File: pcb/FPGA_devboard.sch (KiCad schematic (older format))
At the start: 4 parts

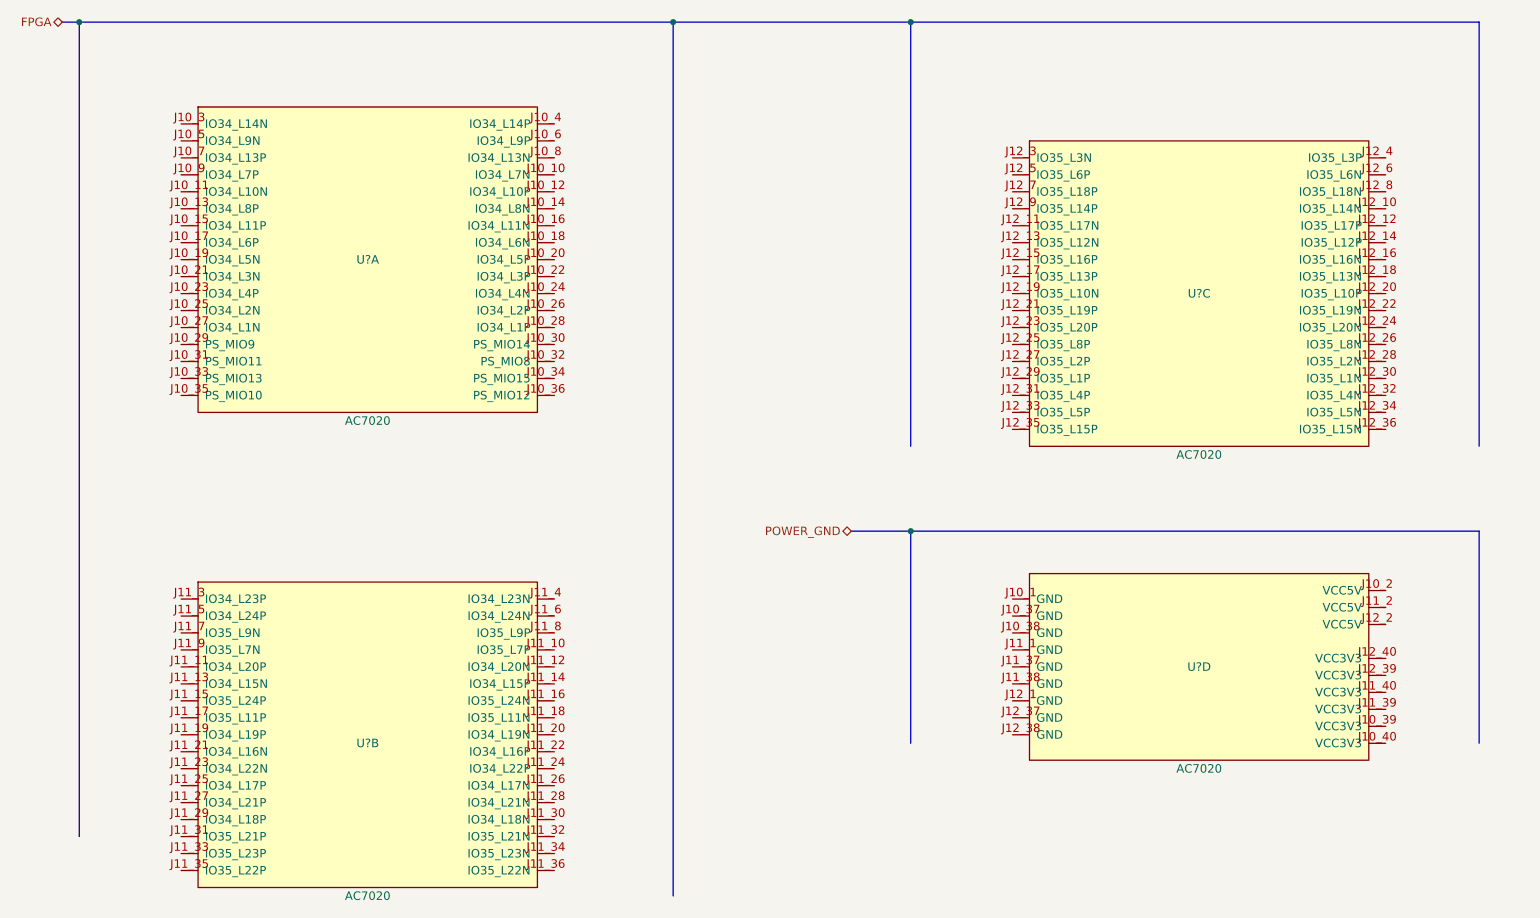
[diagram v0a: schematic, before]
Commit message: Some work done on the whole project
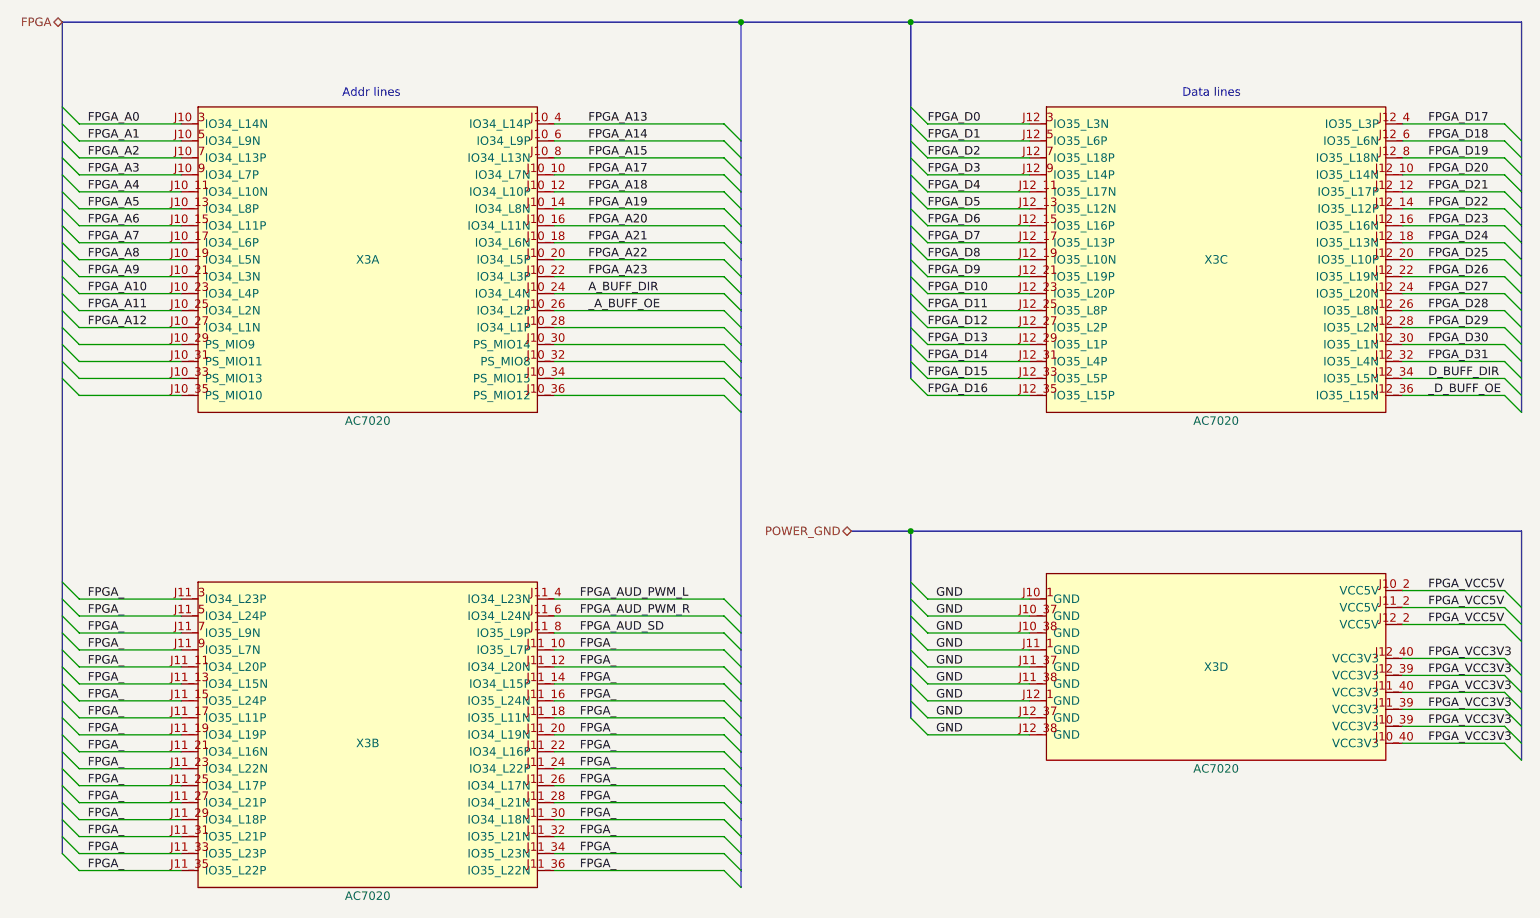
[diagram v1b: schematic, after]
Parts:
- gave numbers to parts that had none: 1
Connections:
- net FPGA_A17: now reaches X3.J10_10 (IO34_L7N)
- net FPGA_A4: now reaches X3.J10_11 (IO34_L10N)
- net FPGA_A18: now reaches X3.J10_12 (IO34_L10P)
- net FPGA_A5: now reaches X3.J10_13 (IO34_L8P)
- net FPGA_A19: now reaches X3.J10_14 (IO34_L8N)
- net FPGA_A6: now reaches X3.J10_15 (IO34_L11P)
- net FPGA_A20: now reaches X3.J10_16 (IO34_L11N)
- net FPGA_A7: now reaches X3.J10_17 (IO34_L6P)
- net FPGA_A21: now reaches X3.J10_18 (IO34_L6N)
- net FPGA_A8: now reaches X3.J10_19 (IO34_L5N)
- net FPGA_A22: now reaches X3.J10_20 (IO34_L5P)
- net FPGA_A9: now reaches X3.J10_21 (IO34_L3N)
- net FPGA_A23: now reaches X3.J10_22 (IO34_L3P)
- net FPGA_A10: now reaches X3.J10_23 (IO34_L4P)
- net A_BUFF_DIR: now reaches X3.J10_24 (IO34_L4N)
- net FPGA_A11: now reaches X3.J10_25 (IO34_L2N)
- net _A_BUFF_OE: now reaches X3.J10_26 (IO34_L2P)
- net FPGA_A12: now reaches X3.J10_27 (IO34_L1N)
- net FPGA_A0: now reaches X3.J10_3 (IO34_L14N)
- net FPGA_A13: now reaches X3.J10_4 (IO34_L14P)
- net FPGA_A1: now reaches X3.J10_5 (IO34_L9N)
- net FPGA_A14: now reaches X3.J10_6 (IO34_L9P)
- net FPGA_A2: now reaches X3.J10_7 (IO34_L13P)
- net FPGA_A15: now reaches X3.J10_8 (IO34_L13N)
- net FPGA_A3: now reaches X3.J10_9 (IO34_L7P)
- net FPGA_: now reaches X3.J11_10 (IO35_L7P)
- net FPGA_: now also X3.J11_11 (IO34_L20P), X3.J11_12 (IO34_L20N), X3.J11_13 (IO34_L15N), X3.J11_14 (IO34_L15P), X3.J11_15 (IO35_L24P), X3.J11_16 (IO35_L24N), X3.J11_17 (IO35_L11P), X3.J11_18 (IO35_L11N), X3.J11_19 (IO34_L19P), X3.J11_20 (IO34_L19N), X3.J11_21 (IO34_L16N), X3.J11_22 (IO34_L16P), X3.J11_23 (IO34_L22N), X3.J11_24 (IO34_L22P), X3.J11_25 (IO34_L17P), X3.J11_26 (IO34_L17N), X3.J11_27 (IO34_L21P), X3.J11_28 (IO34_L21N), X3.J11_29 (IO34_L18P), X3.J11_3 (IO34_L23P), X3.J11_30 (IO34_L18N), X3.J11_31 (IO35_L21P), X3.J11_32 (IO35_L21N), X3.J11_33 (IO35_L23P), X3.J11_34 (IO35_L23N), X3.J11_35 (IO35_L22P), X3.J11_36 (IO35_L22N), X3.J11_5 (IO34_L24P), X3.J11_7 (IO35_L9N), X3.J11_9 (IO35_L7N)
- net FPGA_AUD_PWM_L: now reaches X3.J11_4 (IO34_L23N)
- net FPGA_AUD_PWM_R: now reaches X3.J11_6 (IO34_L24N)
- net FPGA_AUD_SD: now reaches X3.J11_8 (IO35_L9P)
- net FPGA_D20: now reaches X3.J12_10 (IO35_L14N)
- net FPGA_D4: now reaches X3.J12_11 (IO35_L17N)
- net FPGA_D21: now reaches X3.J12_12 (IO35_L17P)
- net FPGA_D5: now reaches X3.J12_13 (IO35_L12N)
- net FPGA_D22: now reaches X3.J12_14 (IO35_L12P)
- net FPGA_D6: now reaches X3.J12_15 (IO35_L16P)
- net FPGA_D23: now reaches X3.J12_16 (IO35_L16N)
- net FPGA_D7: now reaches X3.J12_17 (IO35_L13P)
- net FPGA_D24: now reaches X3.J12_18 (IO35_L13N)
- net FPGA_D8: now reaches X3.J12_19 (IO35_L10N)
- net FPGA_D25: now reaches X3.J12_20 (IO35_L10P)
- net FPGA_D9: now reaches X3.J12_21 (IO35_L19P)
- net FPGA_D26: now reaches X3.J12_22 (IO35_L19N)
- net FPGA_D10: now reaches X3.J12_23 (IO35_L20P)
- net FPGA_D27: now reaches X3.J12_24 (IO35_L20N)
- net FPGA_D11: now reaches X3.J12_25 (IO35_L8P)
- net FPGA_D28: now reaches X3.J12_26 (IO35_L8N)
- net FPGA_D12: now reaches X3.J12_27 (IO35_L2P)
- net FPGA_D29: now reaches X3.J12_28 (IO35_L2N)
- net FPGA_D13: now reaches X3.J12_29 (IO35_L1P)
- net FPGA_D0: now reaches X3.J12_3 (IO35_L3N)
- net FPGA_D30: now reaches X3.J12_30 (IO35_L1N)
- net FPGA_D14: now reaches X3.J12_31 (IO35_L4P)
- net FPGA_D31: now reaches X3.J12_32 (IO35_L4N)
- net FPGA_D15: now reaches X3.J12_33 (IO35_L5P)
- net D_BUFF_DIR: now reaches X3.J12_34 (IO35_L5N)
- net FPGA_D16: now reaches X3.J12_35 (IO35_L15P)
- net _D_BUFF_OE: now reaches X3.J12_36 (IO35_L15N)
- net FPGA_D17: now reaches X3.J12_4 (IO35_L3P)
- net FPGA_D1: now reaches X3.J12_5 (IO35_L6P)
- net FPGA_D18: now reaches X3.J12_6 (IO35_L6N)
- net FPGA_D2: now reaches X3.J12_7 (IO35_L18P)
- net FPGA_D19: now reaches X3.J12_8 (IO35_L18N)
- net FPGA_D3: now reaches X3.J12_9 (IO35_L14P)
- net GND: now reaches X3.J10_1 (GND)
- net GND: now also X3.J10_37 (GND), X3.J10_38 (GND), X3.J11_1 (GND), X3.J11_37 (GND), X3.J11_38 (GND), X3.J12_1 (GND), X3.J12_37 (GND), X3.J12_38 (GND)
- net FPGA_VCC5V: now reaches X3.J10_2 (VCC5V)
- net FPGA_VCC5V: now also X3.J11_2 (VCC5V), X3.J12_2 (VCC5V)
- net FPGA_VCC3V3: now reaches X3.J10_39 (VCC3V3)
- net FPGA_VCC3V3: now also X3.J10_40 (VCC3V3), X3.J11_39 (VCC3V3), X3.J11_40 (VCC3V3), X3.J12_39 (VCC3V3), X3.J12_40 (VCC3V3)
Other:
- note added: "Addr lines"
- note added: "Data lines"
- moved on the sheet: X3C, X3D
